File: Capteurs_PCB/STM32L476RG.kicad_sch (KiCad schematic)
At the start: 1 part, among them U2 STM32L476RGTx

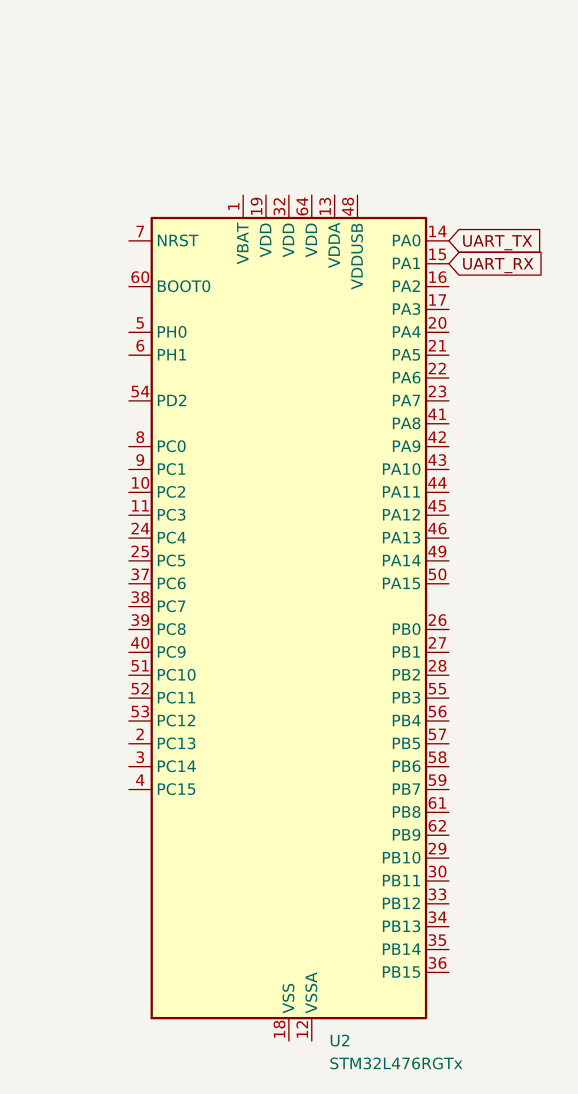
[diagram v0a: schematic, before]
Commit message: pcb update
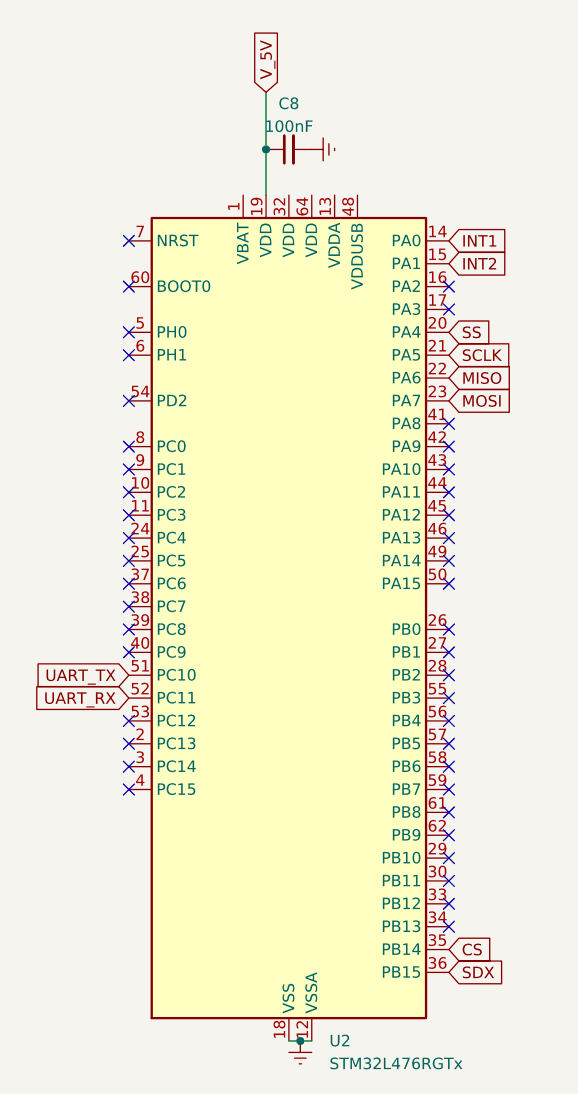
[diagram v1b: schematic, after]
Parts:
- added C8: 100nF, symbol Device:C_Small
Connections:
- net UART_RX: now also U2.52 (PC11); no longer U2.15 (PA1)
- net UART_TX: now also U2.51 (PC10); no longer U2.14 (PA0)
- net Earth: now reaches U2.12 (VSSA)
- net Earth: now also U2.18 (VSS), U2.31 (VSS), U2.47 (VSS), U2.63 (VSS), C8.2
- net V_5V: now reaches U2.19 (VDD)
- net V_5V: now also C8.1
- net SS: now reaches U2.20 (PA4)
- net SCLK: now reaches U2.21 (PA5)
- net MISO: now reaches U2.22 (PA6)
- net MOSI: now reaches U2.23 (PA7)
- net CS: now reaches U2.35 (PB14)
- net SDX: now reaches U2.36 (PB15)
- new net INT1: U2.14 (PA0)
- new net INT2: U2.15 (PA1)
- no-connect marks 0 -> 43
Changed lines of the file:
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@@
 (kicad_sch (version 20230121) (generator eeschema)
   (paper "A4")
-  (global_label "UART_RX" (shape input) (at 157.48 59.69 0) (fields_autoplaced)
-    (effects (font (size 1.27 1.27)) (justify left))
-    (property "Intersheetrefs" "${INTERSHEET_REFS}" (at 168.4896 59.69 0)
-      (effects (font (size 1.27 1.27)) (justify left) hide)
-    )
-  )
-  (global_label "UART_TX" (shape input) (at 157.48 57.15 0) (fields_autoplaced)
-    (effects (font (size 1.27 1.27)) (justify left))
-    (property "Intersheetrefs" "${INTERSHEET_REFS}" (at 168.1872 57.15 0)
+  (junction (at 137.16 46.99) (diameter 0) (color 0 0 0 0)
+  )
+  (junction (at 140.97 146.05) (diameter 0) (color 0 0 0 0)
+  )
+  (no_connect (at 121.92 118.11))
+  (no_connect (at 121.92 82.55))
+  (no_connect (at 121.92 74.93))
+  (no_connect (at 121.92 102.87))
+  (no_connect (at 121.92 100.33))
+  (no_connect (at 157.48 102.87))
+  (no_connect (at 157.48 92.71))
+  (no_connect (at 157.48 87.63))
+  (no_connect (at 157.48 125.73))
+  (no_connect (at 157.48 95.25))
+  (no_connect (at 157.48 118.11))
+  (no_connect (at 121.92 95.25))
+  (no_connect (at 157.48 77.47))
+  (no_connect (at 157.48 107.95))
+  (no_connect (at 121.92 85.09))
+  (no_connect (at 121.92 115.57))
+  (no_connect (at 121.92 113.03))
+  (no_connect (at 157.48 100.33))
+  (no_connect (at 121.92 69.85))
+  (no_connect (at 157.48 113.03))
+  (no_connect (at 121.92 87.63))
+  (no_connect (at 121.92 110.49))
+  (no_connect (at 121.92 57.15))
+  (no_connect (at 157.48 128.27))
+  (no_connect (at 157.48 123.19))
+  (no_connect (at 157.48 90.17))
+  (no_connect (at 121.92 97.79))
+  (no_connect (at 157.48 133.35))
+  (no_connect (at 157.48 130.81))
+  (no_connect (at 121.92 62.23))
+  (no_connect (at 157.48 105.41))
+  (no_connect (at 121.92 80.01))
+  (no_connect (at 157.48 80.01))
+  (no_connect (at 157.48 115.57))
+  (no_connect (at 157.48 64.77))
+  (no_connect (at 157.48 85.09))
+  (no_connect (at 121.92 90.17))
+  (no_connect (at 121.92 67.31))
+  (no_connect (at 157.48 120.65))
+  (no_connect (at 121.92 92.71))
+  (no_connect (at 157.48 62.23))
+  (no_connect (at 157.48 110.49))
+  (no_connect (at 157.48 82.55))
+  (wire (pts (xy 140.97 146.05) (xy 142.24 146.05))
+    (stroke (width 0) (type default))
+  )
+  (wire (pts (xy 139.7 146.05) (xy 140.97 146.05))
+    (stroke (width 0) (type default))
+  )
+  (wire (pts (xy 137.16 46.99) (xy 137.16 52.07))
+    (stroke (width 0) (type default))
+  )
+  (wire (pts (xy 137.16 40.64) (xy 137.16 46.99))
+    (stroke (width 0) (type default))
+  )
+  (global_label "INT1" (shape input) (at 157.48 57.15 0) (fields_autoplaced)
+    (effects (font (size 1.27 1.27)) (justify left))
+    (property "Intersheetrefs" "${INTERSHEET_REFS}" (at 164.4982 57.15 0)
+      (effects (font (size 1.27 1.27)) (justify left) hide)
+    )
+  )
+  (global_label "INT2" (shape input) (at 157.48 59.69 0) (fields_autoplaced)
+    (effects (font (size 1.27 1.27)) (justify left))
+    (property "Intersheetrefs" "${INTERSHEET_REFS}" (at 164.4982 59.69 0)
+      (effects (font (size 1.27 1.27)) (justify left) hide)
+    )
+  )
+  (global_label "SDX" (shape input) (at 157.48 138.43 0) (fields_autoplaced)
+    (effects (font (size 1.27 1.27)) (justify left))
+    (property "Intersheetrefs" "${INTERSHEET_REFS}" (at 164.0748 138.43 0)
+      (effects (font (size 1.27 1.27)) (justify left) hide)
+    )
+  )
+  (global_label "UART_RX" (shape input) (at 121.92 107.95 180) (fields_autoplaced)
+    (effects (font (size 1.27 1.27)) (justify right))
+    (property "Intersheetrefs" "${INTERSHEET_REFS}" (at 110.9104 107.95 0)
+      (effects (font (size 1.27 1.27)) (justify right) hide)
+    )
+  )
+  (global_label "CS" (shape input) (at 157.48 135.89 0) (fields_autoplaced)
+    (effects (font (size 1.27 1.27)) (justify left))
+    (property "Intersheetrefs" "${INTERSHEET_REFS}" (at 162.8653 135.89 0)
+      (effects (font (size 1.27 1.27)) (justify left) hide)
+    )
+  )
+  (global_label "UART_TX" (shape input) (at 121.92 105.41 180) (fields_autoplaced)
+    (effects (font (size 1.27 1.27)) (justify right))
+    (property "Intersheetrefs" "${INTERSHEET_REFS}" (at 111.2128 105.41 0)
+      (effects (font (size 1.27 1.27)) (justify right) hide)
+    )
+  )
+  (global_label "V_5V" (shape input) (at 137.16 40.64 90) (fields_autoplaced)
+    (effects (font (size 1.27 1.27)) (justify left))
+    (property "Intersheetrefs" "${INTERSHEET_REFS}" (at 137.16 33.3799 90)
+      (effects (font (size 1.27 1.27)) (justify left) hide)
+    )
+  )
+  (global_label "SCLK" (shape input) (at 157.48 69.85 0) (fields_autoplaced)
+    (effects (font (size 1.27 1.27)) (justify left))
+    (property "Intersheetrefs" "${INTERSHEET_REFS}" (at 165.1634 69.85 0)
+      (effects (font (size 1.27 1.27)) (justify left) hide)
+    )
+  )
+  (global_label "MOSI" (shape input) (at 157.48 74.93 0) (fields_autoplaced)
+    (effects (font (size 1.27 1.27)) (justify left))
+    (property "Intersheetrefs" "${INTERSHEET_REFS}" (at 164.982 74.93 0)
+      (effects (font (size 1.27 1.27)) (justify left) hide)
+    )
+  )
+  (global_label "MISO" (shape input) (at 157.48 72.39 0) (fields_autoplaced)
+    (effects (font (size 1.27 1.27)) (justify left))
+    (property "Intersheetrefs" "${INTERSHEET_REFS}" (at 164.982 72.39 0)
+      (effects (font (size 1.27 1.27)) (justify left) hide)
+    )
+  )
+  (global_label "SS" (shape input) (at 157.48 67.31 0) (fields_autoplaced)
+    (effects (font (size 1.27 1.27)) (justify left))
+    (property "Intersheetrefs" "${INTERSHEET_REFS}" (at 162.8048 67.31 0)
       (effects (font (size 1.27 1.27)) (justify left) hide)
     )
@@
         )
       )
+    )
+  )
+  (symbol (lib_id "power:Earth") (at 142.24 46.99 90) (unit 1)
+    (in_bom yes) (on_board yes) (dnp no) (fields_autoplaced)
+    (property "Reference" "#PWR06" (at 148.59 46.99 0)
+      (effects (font (size 1.27 1.27)) hide)
+    )
+    (property "Value" "Earth" (at 146.05 46.99 0)
+      (effects (font (size 1.27 1.27)) hide)
+    )
+    (property "Footprint" "" (at 142.24 46.99 0)
+      (effects (font (size 1.27 1.27)) hide)
+    )
+    (property "Datasheet" "~" (at 142.24 46.99 0)
+      (effects (font (size 1.27 1.27)) hide)
+    )
+    (pin "1")
+    (instances
+      (project "Capteurs_PCB"
+        (path "/1101af8f-9425-4102-9245-339dc54562bf/484fed71-765a-4020-a5ac-867b14a93f63"
+          (reference "#PWR06") (unit 1)
+        )
+      )
+    )
+  )
+  (symbol (lib_id "Device:C_Small") (at 139.7 46.99 90) (unit 1)
+    (in_bom yes) (on_board yes) (dnp no) (fields_autoplaced)
+    (property "Reference" "C8" (at 139.7063 41.91 90)
+      (effects (font (size 1.27 1.27)))
+    )
+    (property "Value" "100nF" (at 139.7063 44.45 90)
+      (effects (font (size 1.27 1.27)))
+    )
+    (property "Footprint" "" (at 139.7 46.99 0)
+      (effects (font (size 1.27 1.27)) hide)
+    )
+    (property "Datasheet" "~" (at 139.7 46.99 0)
+      (effects (font (size 1.27 1.27)) hide)
+    )
+    (pin "1")
+    (pin "2")
+    (instances
+      (project "Capteurs_PCB"
+        (path "/1101af8f-9425-4102-9245-339dc54562bf/484fed71-765a-4020-a5ac-867b14a93f63"
+          (reference "C8") (unit 1)
+        )
+      )
+    )
+  )
+  (symbol (lib_id "power:Earth") (at 140.97 146.05 0) (unit 1)
+    (in_bom yes) (on_board yes) (dnp no) (fields_autoplaced)
+    (property "Reference" "#PWR08" (at 140.97 152.4 0)
+      (effects (font (size 1.27 1.27)) hide)
+    )
+    (property "Value" "Earth" (at 140.97 149.86 0)
+      (effects (font (size 1.27 1.27)) hide)
+    )
+    (property "Footprint" "" (at 140.97 146.05 0)
+      (effects (font (size 1.27 1.27)) hide)
+    )
+    (property "Datasheet" "~" (at 140.97 146.05 0)
+      (effects (font (size 1.27 1.27)) hide)
+    )
+    (pin "1")
+    (instances
+      (project "Capteurs_PCB"
+        (path "/1101af8f-9425-4102-9245-339dc54562bf/484fed71-765a-4020-a5ac-867b14a93f63"
+          (reference "#PWR08") (unit 1)
+        )
+      )
